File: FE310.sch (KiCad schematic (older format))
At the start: 45 parts, among them Q2 SSM3K35AMFV, Q3 SSM3K35AMFV, SW1 NP_TACTILE_SWITCH, SW2 TACTILE_SWITCH, U4 FE310-G000, U5 IS25LP128-JBLE, Y1 16MHz

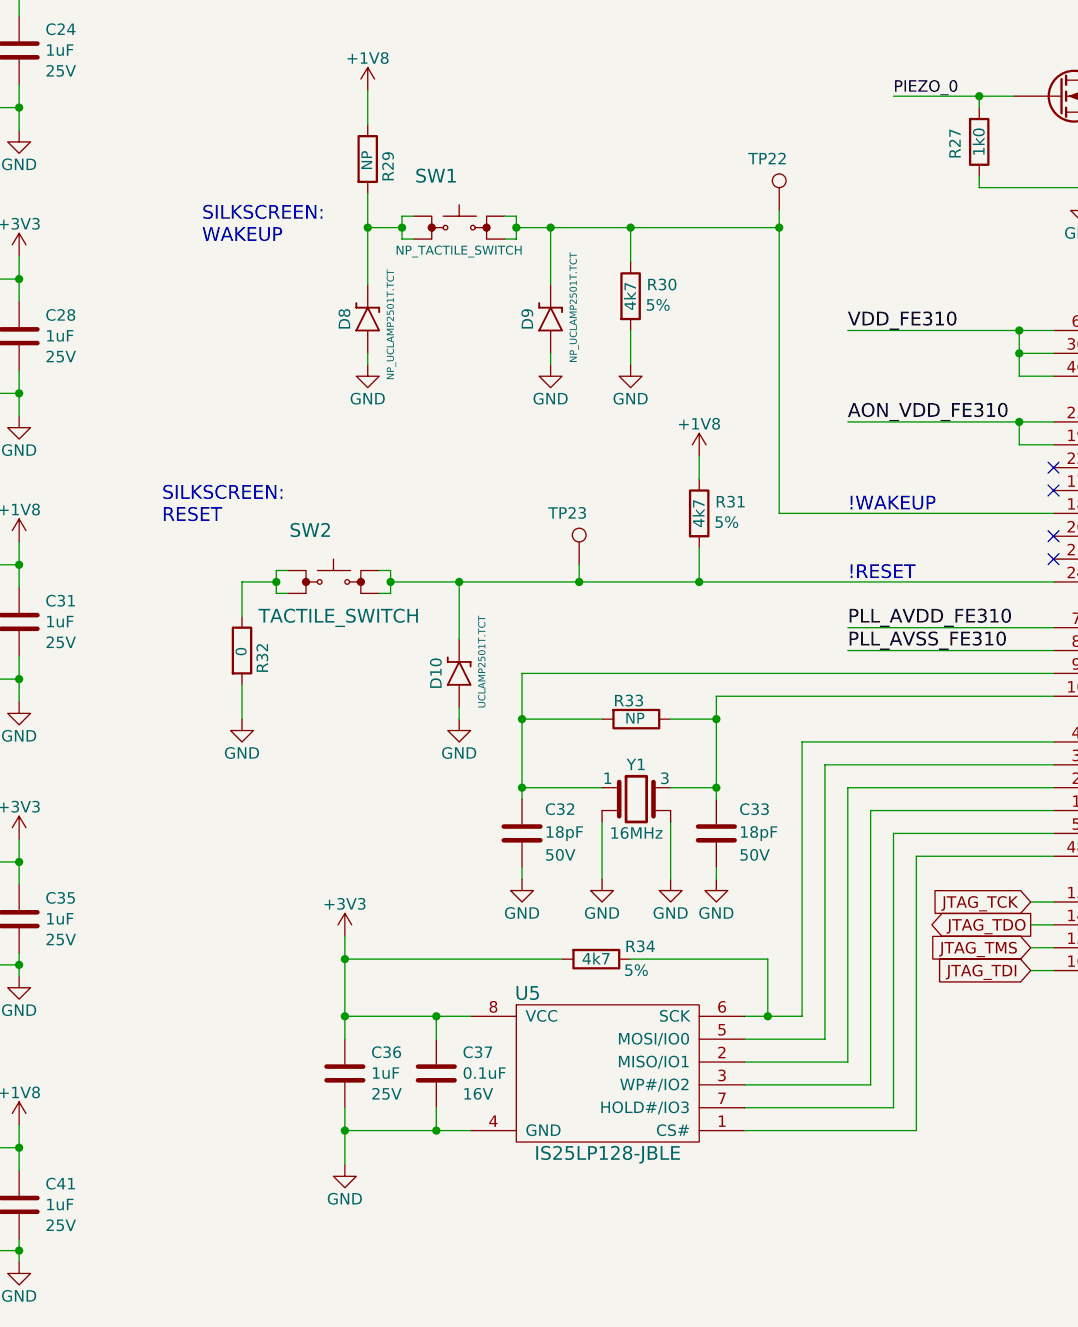
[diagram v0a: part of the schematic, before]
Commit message: automated commit
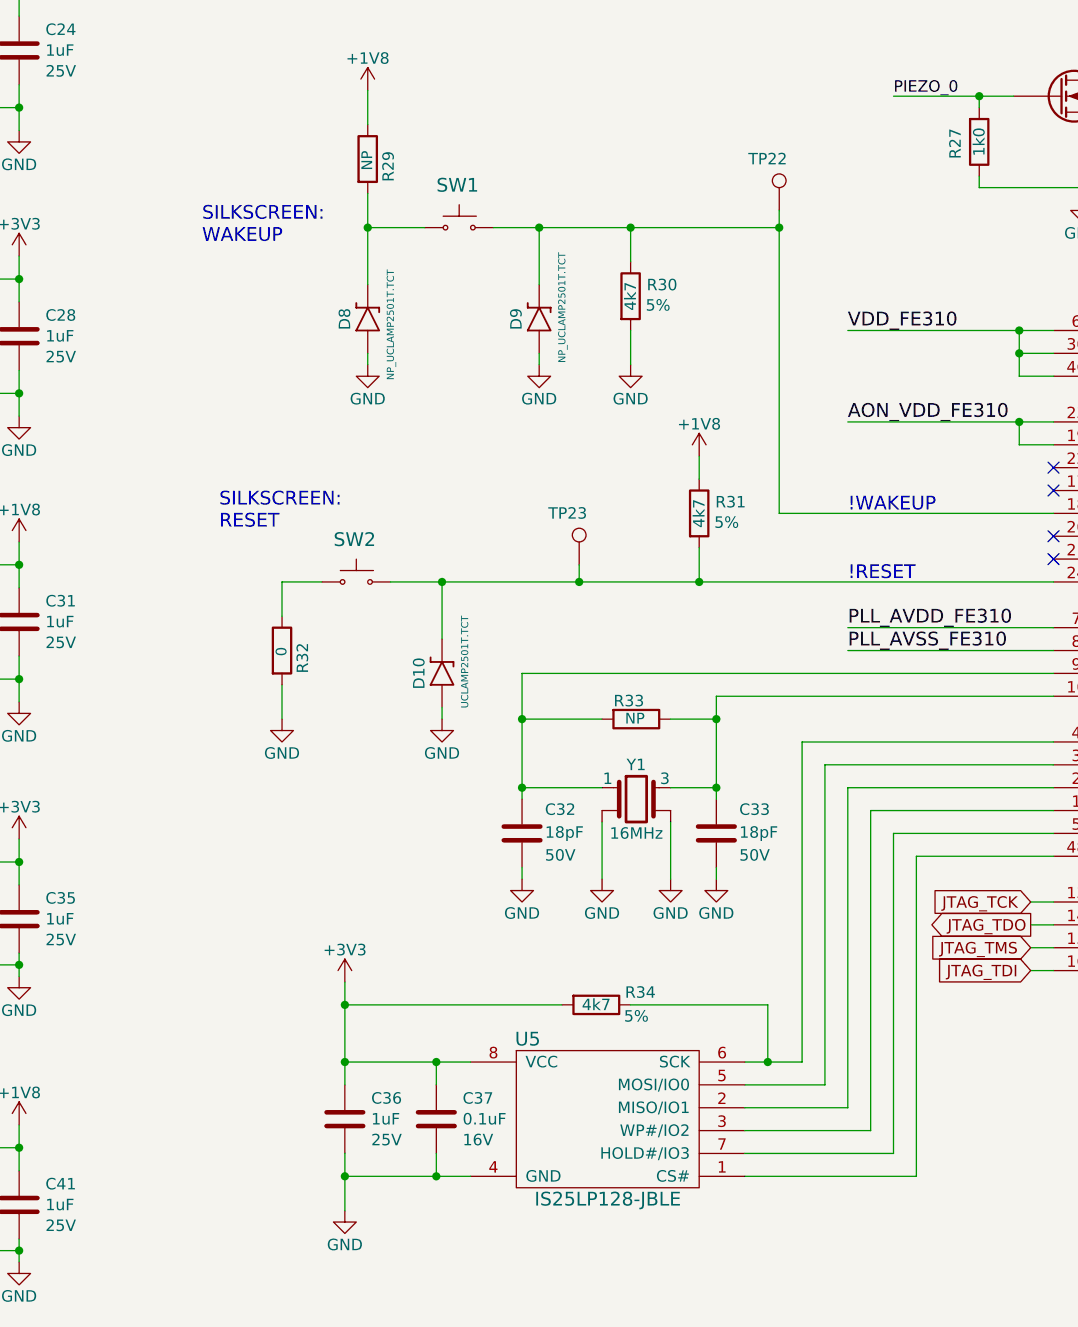
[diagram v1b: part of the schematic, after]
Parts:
- removed SW1: NP_TACTILE_SWITCH, CUSTOM:TACTILE_SWITCH, symbol custom:TACTILE_SWITCH
- removed SW2: TACTILE_SWITCH, CUSTOM:TACTILE_SWITCH, symbol custom:TACTILE_SWITCH
- added SW1, SW2: TACTILE_SWITCH_SMALL, custom:TACTILE_SWITCH_SMALL, symbol custom:TACTILE_SWITCH_SMALL
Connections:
- net at D9.1 (K), R30.1, TP22.1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: now also SW1.2
- net at D10.1 (K), R31.2, TP23.1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: now also SW2.2
- net at R32.1: now also SW2.1
- net at D8.1 (K), R29.2: now also SW1.1
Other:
- moved on the sheet: C36, C37, D10, D9, R32, R34, U5
